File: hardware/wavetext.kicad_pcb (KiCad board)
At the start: 2 copper layers, 150 x 30 mm, 29 parts, among them IC0 ATTINY2313A-S, P1 CONN_6, Q1 OPTO_NPN, SW0 DUAL_SWITCH_INV, SW1 SW_PUSH, U0 ST L78L33ACUTR

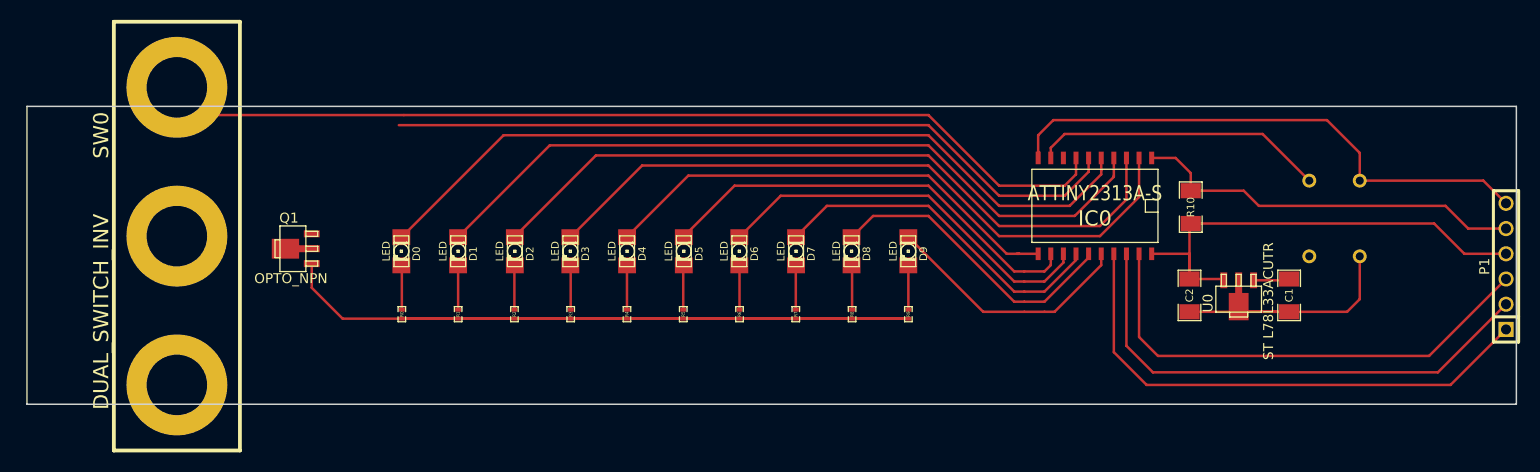
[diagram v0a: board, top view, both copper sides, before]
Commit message: rearranged pcb parts
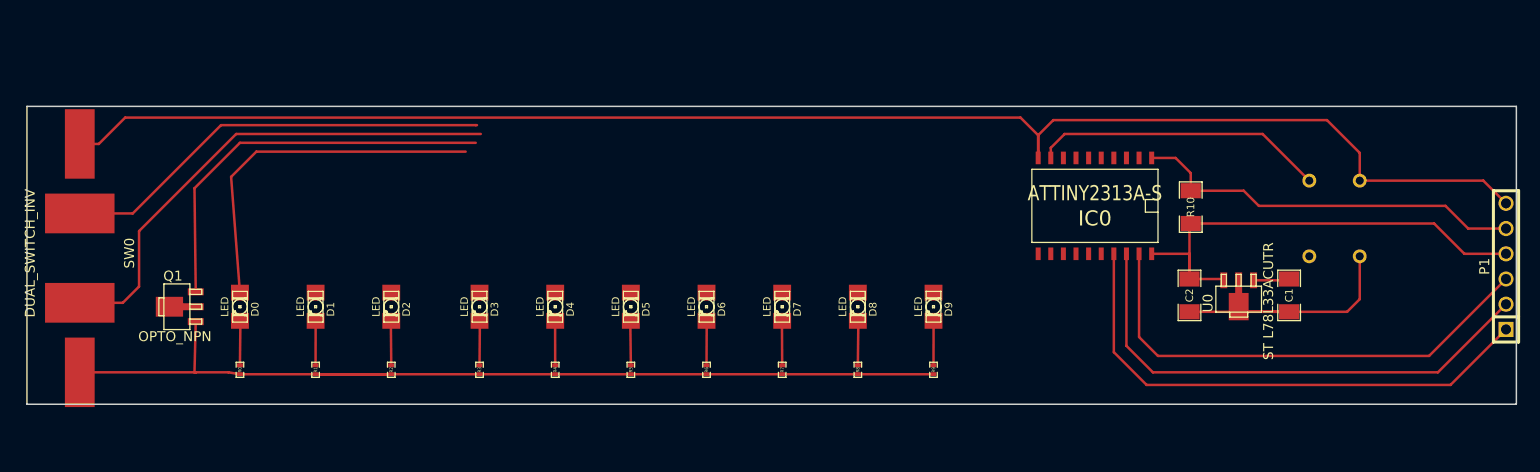
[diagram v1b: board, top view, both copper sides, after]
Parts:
- SW0: footprint 3PIN_6mm -> Wackelschalter
- moved R0 17.2 mm to (171.4, 176.5)
- moved D0 17.2 mm to (171.4, 170.2)
- moved SW0 16.8 mm to (155.3, 176.8)
- moved R1 15.4 mm to (179.1, 176.5)
- moved D1 15.4 mm to (179.1, 170.2)
- moved D2 13.6 mm to (186.7, 170.2)
- moved R2 13.6 mm to (186.7, 176.5)
- moved Q1 13.1 mm to (165.1, 170.2)
- moved R3 10.8 mm to (195.6, 176.5)
- moved D3 10.7 mm to (195.6, 170.2)
- moved D4 9.14 mm to (203.2, 170.2)
- moved R4 9.14 mm to (203.2, 176.5)
- moved D5 7.73 mm to (210.8, 170.2)
- moved R5 7.69 mm to (210.8, 176.5)
- moved R6 6.51 mm to (218.4, 176.5)
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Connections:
- IC0 pad 6: N-0000019 (its old number) -> N-0000017
- SW0 pad 1: N-0000019 (its old number) -> GND
- SW0 pad 2: GND -> N-0000017
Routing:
- net N-0000010: track 76.3 -> 0.00 mm
- net N-0000019 (its old number): track 74.8 -> 0.00 mm
- net GND: track 212.9 -> 286.7 mm
- net N-000009: track 73.3 -> 0.00 mm
- net N-000008: track 68.7 -> 0.00 mm
- net N-0000018: track 96.8 -> 43.7 mm
- net N-0000017: track 0.00 -> 50.7 mm
- net N-000001: track 47.5 -> 0.00 mm
- net N-0000011: track 80.6 -> 36.4 mm
- net N-000007: track 44.1 -> 0.00 mm
- net N-0000012: track 0.00 -> 40.7 mm
- net N-000006: track 39.6 -> 0.00 mm
- net N-000005: track 35.0 -> 0.00 mm
- net N-000004: track 30.5 -> 0.00 mm
- net N-000003: track 25.6 -> 0.00 mm
